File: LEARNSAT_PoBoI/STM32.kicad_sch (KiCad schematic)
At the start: 24 parts, among them U401 LP5907SNX-3.3, U402 74AC14MTCX, U403 ISL3259EIRZ, U404 STM32F103RET6, U405 LTC4304CMS#PBF, Y401 ABS07-166-32.768KHZ-T

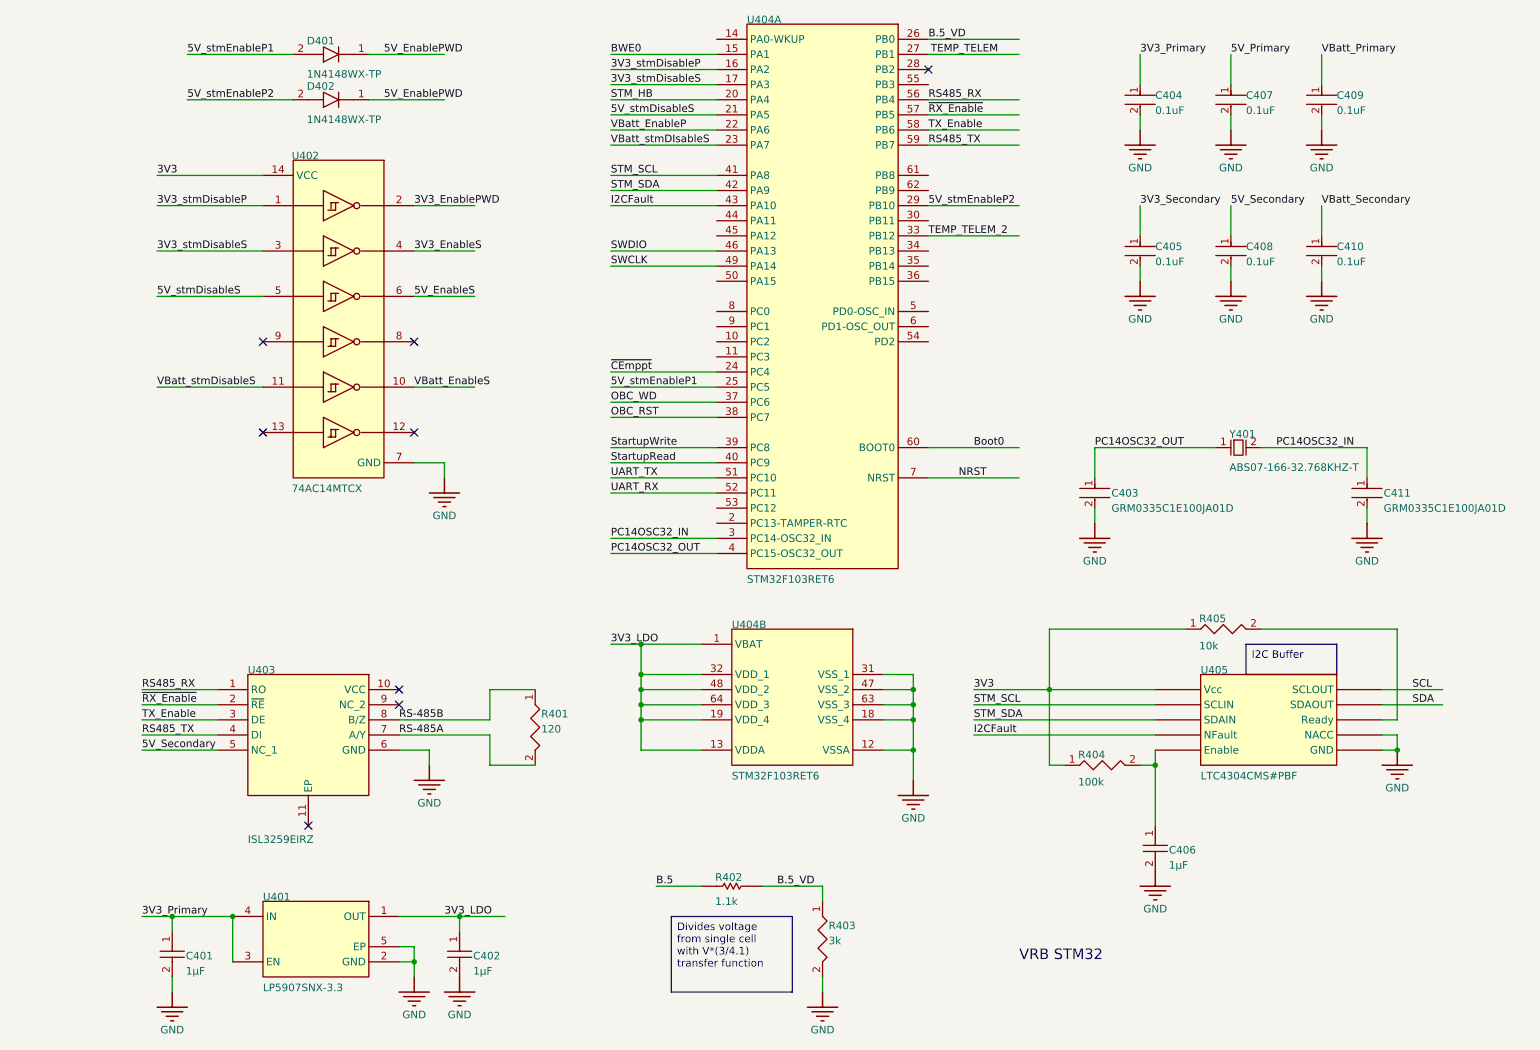
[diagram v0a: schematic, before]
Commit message: Add files via upload
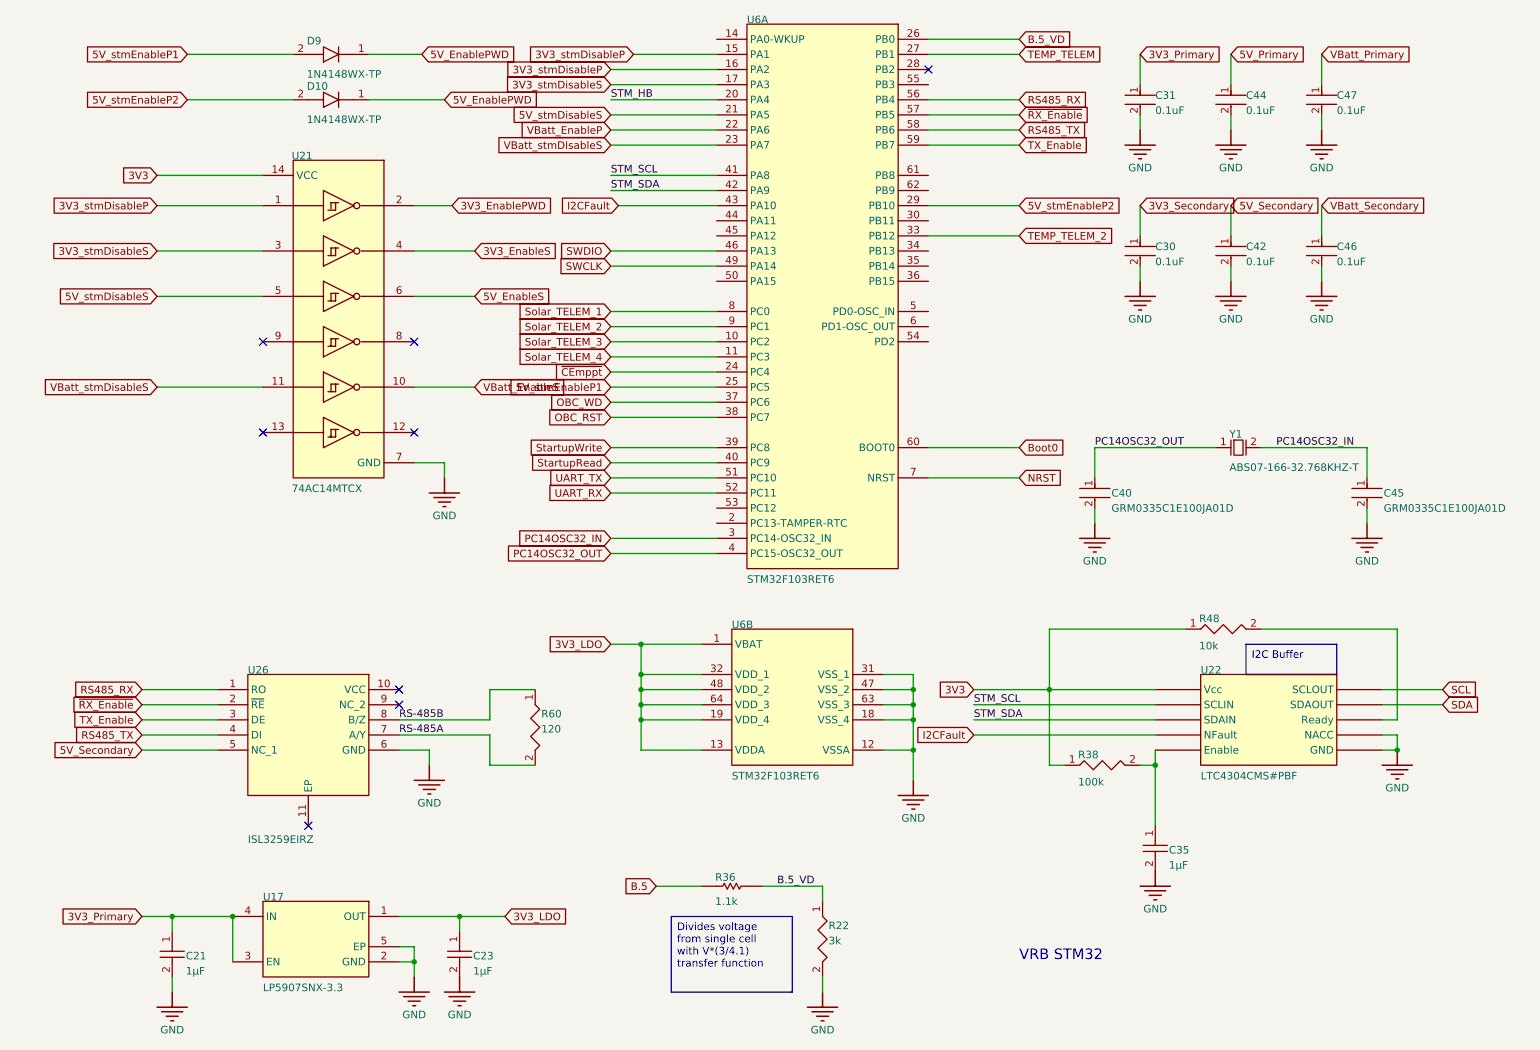
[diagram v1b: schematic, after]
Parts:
- C21: renamed from C401; footprint Capacitor_SMD:C_0201_0603Metric -> FP-CC0201-BA-IPC_A
- C23: renamed from C402; footprint Capacitor_SMD:C_0201_0603Metric -> FP-CC0201-BA-IPC_A
- C30: renamed from C405; footprint Capacitor_SMD:C_0603_1608Metric -> FP-C0603-CJ-MFG
- C31: renamed from C404; footprint Capacitor_SMD:C_0603_1608Metric -> FP-C0603-CJ-MFG
- C35: renamed from C406; footprint Capacitor_SMD:C_0603_1608Metric -> CAPC1608X94X35NL15T15
- C40: renamed from C403; footprint Capacitor_SMD:C_0201_0603Metric -> FP-GRM033-0_03-IPC_A
- C42: renamed from C408; footprint Capacitor_SMD:C_0603_1608Metric -> FP-C0603-CJ-MFG
- C44: renamed from C407; footprint Capacitor_SMD:C_0603_1608Metric -> FP-C0603-CJ-MFG
- C45: renamed from C411; footprint Capacitor_SMD:C_0201_0603Metric -> FP-GRM033-0_03-IPC_A
- C46: renamed from C410; footprint Capacitor_SMD:C_0603_1608Metric -> FP-C0603-CJ-MFG
- C47: renamed from C409; footprint Capacitor_SMD:C_0603_1608Metric -> FP-C0603-CJ-MFG
- D10: renamed from D402; footprint Diode_SMD:D_SOD-323 -> 1N4148WX-TP-Footprint-1
- D9: renamed from D401; footprint Diode_SMD:D_SOD-323 -> 1N4148WX-TP-Footprint-1
- R22: renamed from R403; footprint Resistor_SMD:R_0402_1005Metric -> RESC0402(1005)_L
- R36: renamed from R402; footprint Resistor_SMD:R_0402_1005Metric -> RESC1005X40X25NL05T10
- R38: renamed from R404; footprint Resistor_SMD:R_1206_3216Metric -> RESC3216X60X45ML15T20
- R48: renamed from R405; footprint Resistor_SMD:R_0603_1608Metric -> RESC1608X55X25ML10T15
- R60: renamed from R401; footprint Resistor_SMD:R_0603_1608Metric -> RESC0603(1608)_L
- U17: renamed from U401; footprint LP5907SNX-3.3:IC_TPS7A0230PDQNR -> TI-DQN4-480X480TP_V
- U21: renamed from U402; footprint 74AC14MTCX:SOP65P640X120-14N -> FP-948G-MFG
- U22: renamed from U405; footprint LTC4304CMS_PBF:MSOP-10_MS -> LTC4304CMS#PBF-Footprint-1
- U26: renamed from U403; footprint ISL3259EIRZ-T:SON50P300X300X100-11N -> ISL3259EIRZ-Footprint-1
- U6: renamed from U404; footprint KiCad:QFP50P1200X1200X160-64N -> STM-LQFP64_N
- Y1: renamed from Y401; footprint ABS07-166-32.768KHZ-T:XTAL_ABS07-166-32.768KHZ-T -> EPSON-FC-135_V
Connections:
- net BWE0 is gone; now on net 3V3_stmDisableP: U6.15 (PA1)
- net RS485_TX: now also U6.58 (PB6); no longer U6.59 (PB7)
- net TX_Enable: now also U6.59 (PB7); no longer U6.58 (PB6)
- net Solar_TELEM_3: now reaches U6.10 (PC2)
- net Solar_TELEM_4: now reaches U6.11 (PC3)
- net Solar_TELEM_1: now reaches U6.8 (PC0)
- net Solar_TELEM_2: now reaches U6.9 (PC1)
